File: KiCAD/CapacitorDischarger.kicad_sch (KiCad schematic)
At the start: 44 parts, among them J1 SLB4-G-21, J2 SLB4-G-22, J3 MKDS5/2-9.5, J4 MKDS5/2-9.5, J5 DVM_Connector, Q1 MPSA42, Q2 STP10NK80Z 800V 9A

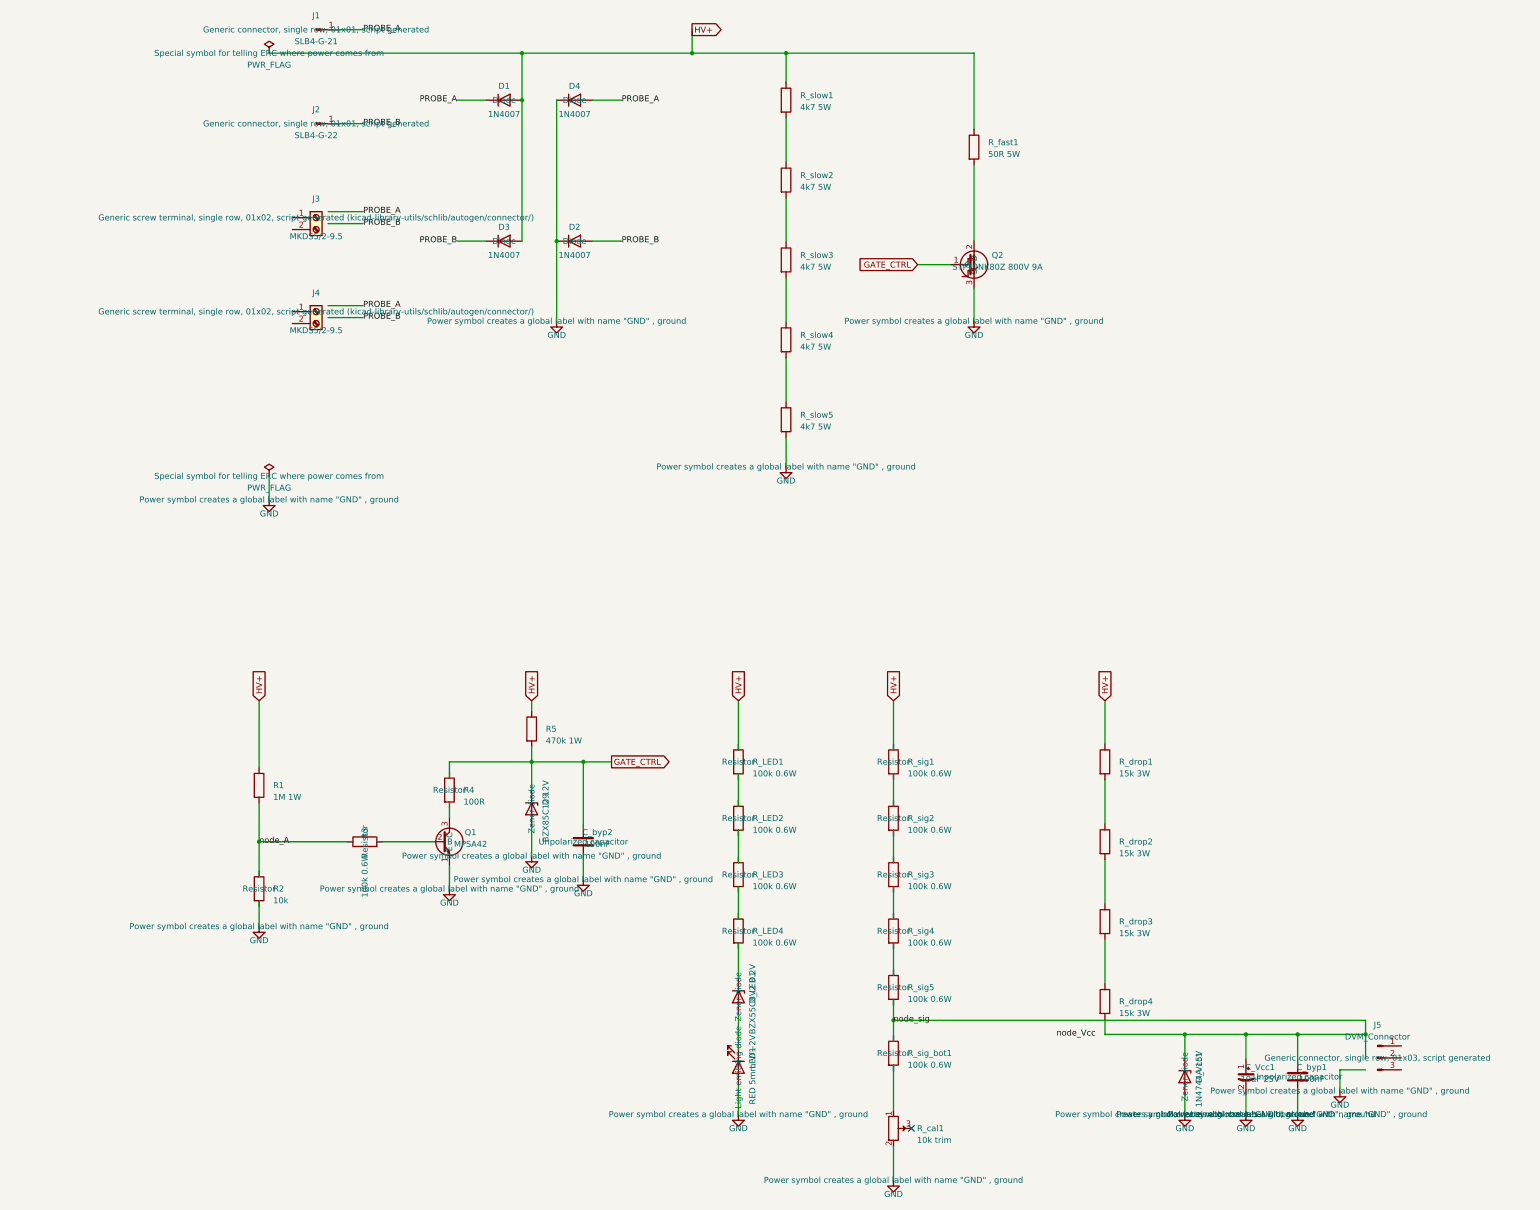
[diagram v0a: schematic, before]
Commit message: KiCAD processing
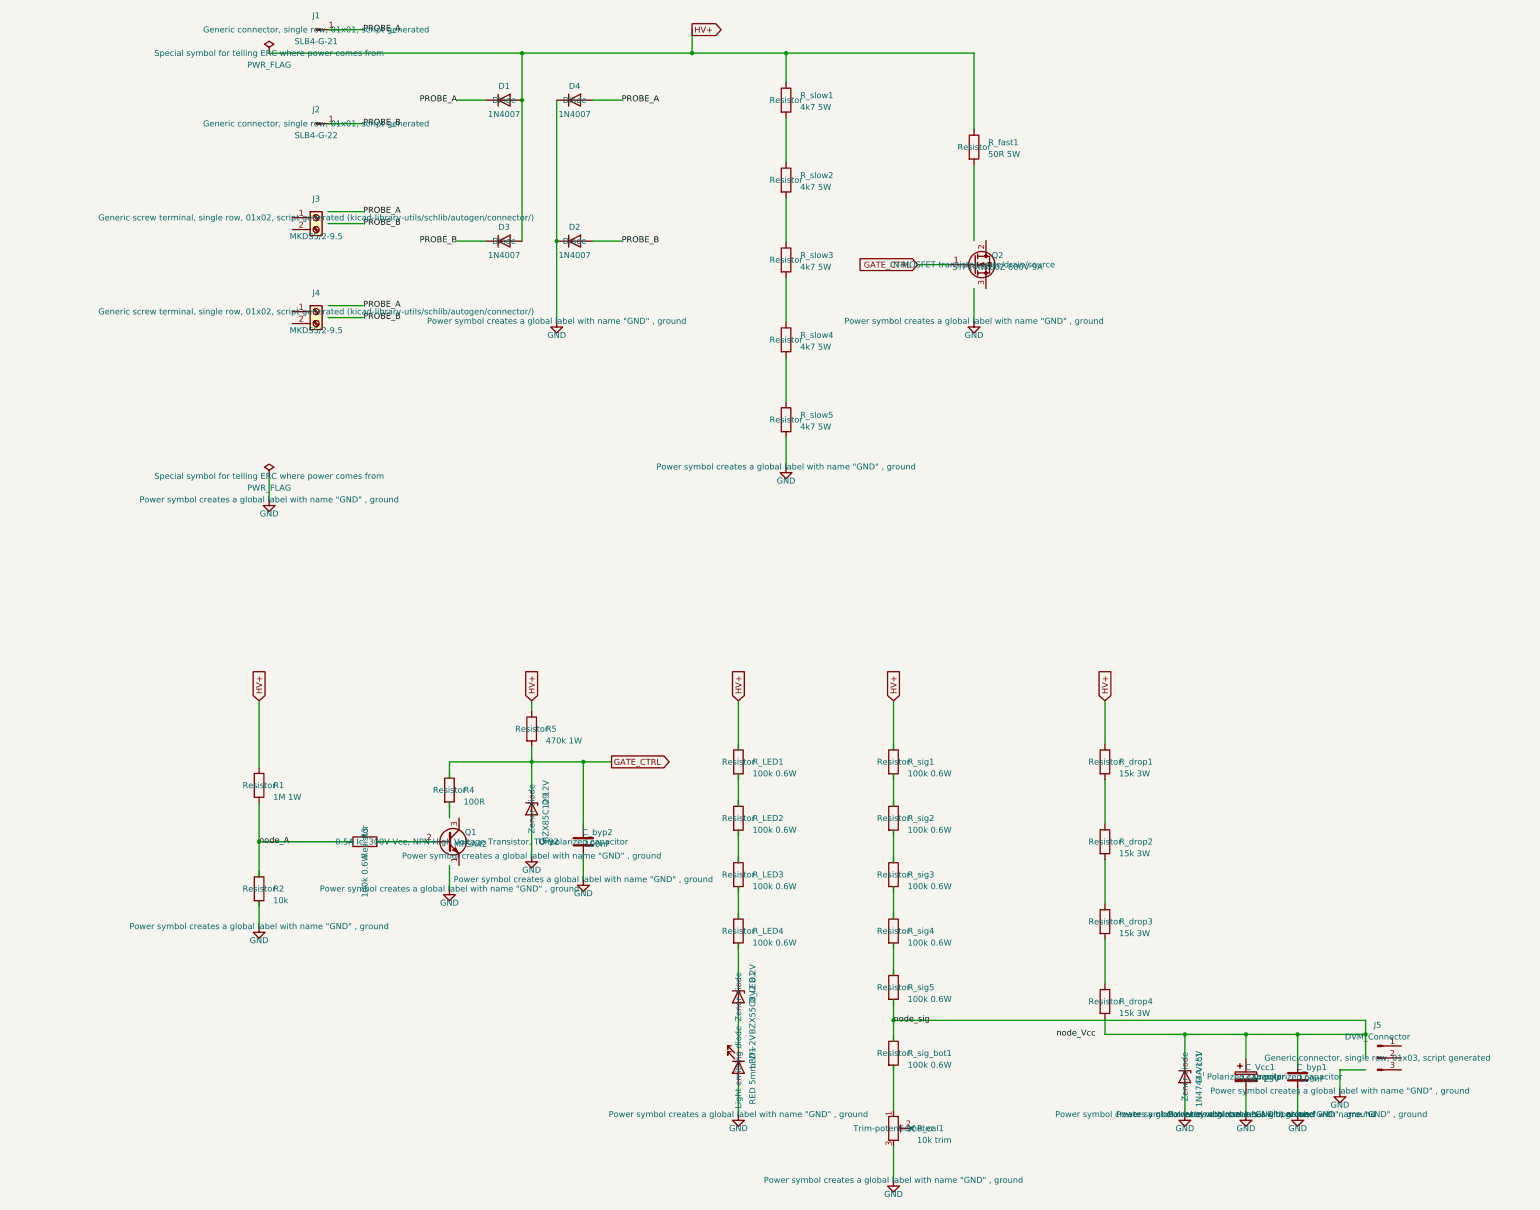
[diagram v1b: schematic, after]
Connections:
- net GND: now also R_cal1.3; no longer Q1.1 (E), Q2.3 (S), R_cal1.2
- net at R_fast1.2: no longer Q2.2 (D)
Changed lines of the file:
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@@
 			)
 		)
-		(property "Description" ""
+		(property "Description" "Resistor"
 			(at 170.18 47.28 0)
 			(show_name no)
@@
 			)
 		)
-		(property "Description" ""
+		(property "Description" "Resistor"
 			(at 170.18 64.28 0)
 			(show_name no)
@@
 			)
 		)
-		(property "Description" ""
+		(property "Description" "Resistor"
 			(at 170.18 81.28 0)
 			(show_name no)
@@
 			)
 		)
-		(property "Description" ""
+		(property "Description" "Resistor"
 			(at 170.18 98.28 0)
 			(show_name no)
@@
 			)
 		)
-		(property "Description" ""
+		(property "Description" "Resistor"
 			(at 170.18 115.28 0)
 			(show_name no)
@@
 			)
 		)
-		(property "Description" ""
+		(property "Description" "Resistor"
 			(at 210.18 57.28 0)
 			(show_name no)
@@
 			)
 		)
-		(property "Description" ""
+		(property "Description" "N-MOSFET transistor, gate/drain/source"
 			(at 210.18 82.28 0)
 			(show_name no)
@@
 			)
 		)
-		(pin "G"
+		(pin "3"
 		)
-		(pin "D"
+		(pin "1"
 		)
-		(pin "S"
+		(pin "2"
 		)
 		(instances
@@
 			)
 		)
-		(property "Description" ""
+		(property "Description" "Resistor"
 			(at 58.04 193.09 0)
 			(show_name no)
@@
 			)
 		)
-		(property "Datasheet" ""
+		(property "Datasheet" "http://www.onsemi.com/pub_link/Collateral/MPSA42-D.PDF"
 			(at 8.04 -6.91 0)
 			(hide yes)
@@
 			)
 		)
-		(property "Description" ""
+		(property "Description" "0.5A Ic, 300V Vce, NPN High Voltage Transistor, TO-92"
 			(at 98.04 205.09 0)
 			(show_name no)
@@
 			)
 		)
-		(pin "B"
+		(property "Sim.Device" "NPN"
+			(at 98.04 205.09 0)
+			(hide yes)
+			(show_name no)
+			(do_not_autoplace no)
+			(effects
+				(font
+					(size 1.27 1.27)
+				)
+			)
 		)
-		(pin "C"
+		(property "Sim.Pins" "1=E 2=B 3=C"
+			(at 98.04 205.09 0)
+			(hide yes)
+			(show_name no)
+			(do_not_autoplace no)
+			(effects
+				(font
+					(size 1.27 1.27)
+				)
+			)
+		)
+		(pin "2"
 		)
-		(pin "E"
+		(pin "3"
+		)
+		(pin "1"
 		)
 		(instances
@@
 			)
 		)
-		(property "Description" ""
+		(property "Description" "Resistor"
 			(at 116.04 181.09 0)
 			(show_name no)
@@
 			)
 		)
-		(property "Description" ""
+		(property "Description" "Trim-potentiometer"
 			(at 193.04 266.09 0)
 			(show_name no)
@@
 			)
 		)
+		(property "Sim.Device" "R"
+			(at 193.04 266.09 0)
+			(hide yes)
+			(show_name no)
+			(do_not_autoplace no)
+			(effects
+				(font
+					(size 1.27 1.27)
+				)
+			)
+		)
+		(property "Sim.Type" "POT"
+			(at 193.04 266.09 0)
+			(hide yes)
+			(show_name no)
+			(do_not_autoplace no)
+			(effects
+				(font
+					(size 1.27 1.27)
+				)
+			)
+		)
+		(property "Sim.Pins" "1=r0 2=wiper 3=r1"
+			(at 193.04 266.09 0)
+			(hide yes)
+			(show_name no)
+			(do_not_autoplace no)
+			(effects
+				(font
+					(size 1.27 1.27)
+				)
+			)
+		)
 		(pin "1"
 		)
@@
 			)
 		)
-		(property "Description" ""
+		(property "Description" "Resistor"
 			(at 238.04 188.09 0)
 			(show_name no)
@@
 			)
 		)
-		(property "Description" ""
+		(property "Description" "Resistor"
 			(at 238.04 205.09 0)
 			(show_name no)
@@
 			)
 		)
-		(property "Description" ""
+		(property "Description" "Resistor"
 			(at 238.04 222.09 0)
 			(show_name no)
@@
 			)
 		)
-		(property "Description" ""
+		(property "Description" "Resistor"
 			(at 238.04 239.09 0)
 			(show_name no)
@@
 			)
 		)
-		(property "Description" ""
+		(property "Description" "Polarized capacitor"
 			(at 268.04 255.09 0)
 			(show_name no)
